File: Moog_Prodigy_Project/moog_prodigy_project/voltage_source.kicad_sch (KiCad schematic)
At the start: 19 parts, among them T1 230 VAC/ 15VAC 1.5A 22W, U24 L78L12, U25 L79L12

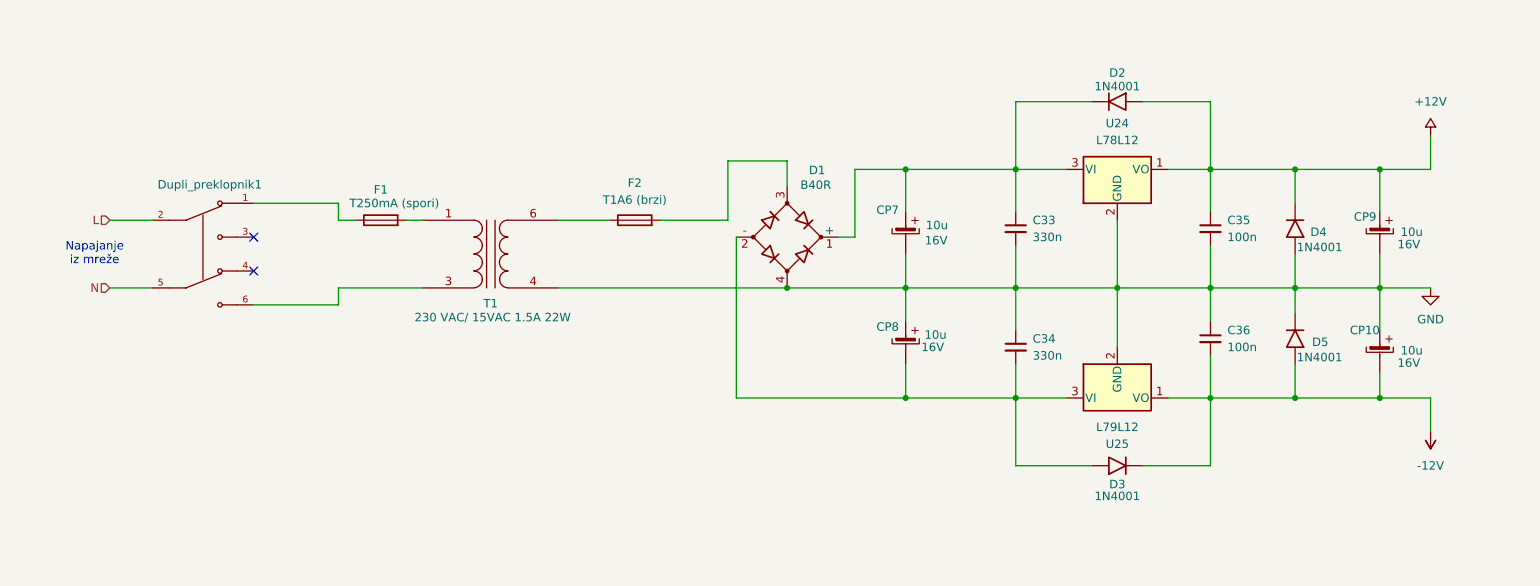
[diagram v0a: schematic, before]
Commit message: MOOG prodigy final 03.07.2026
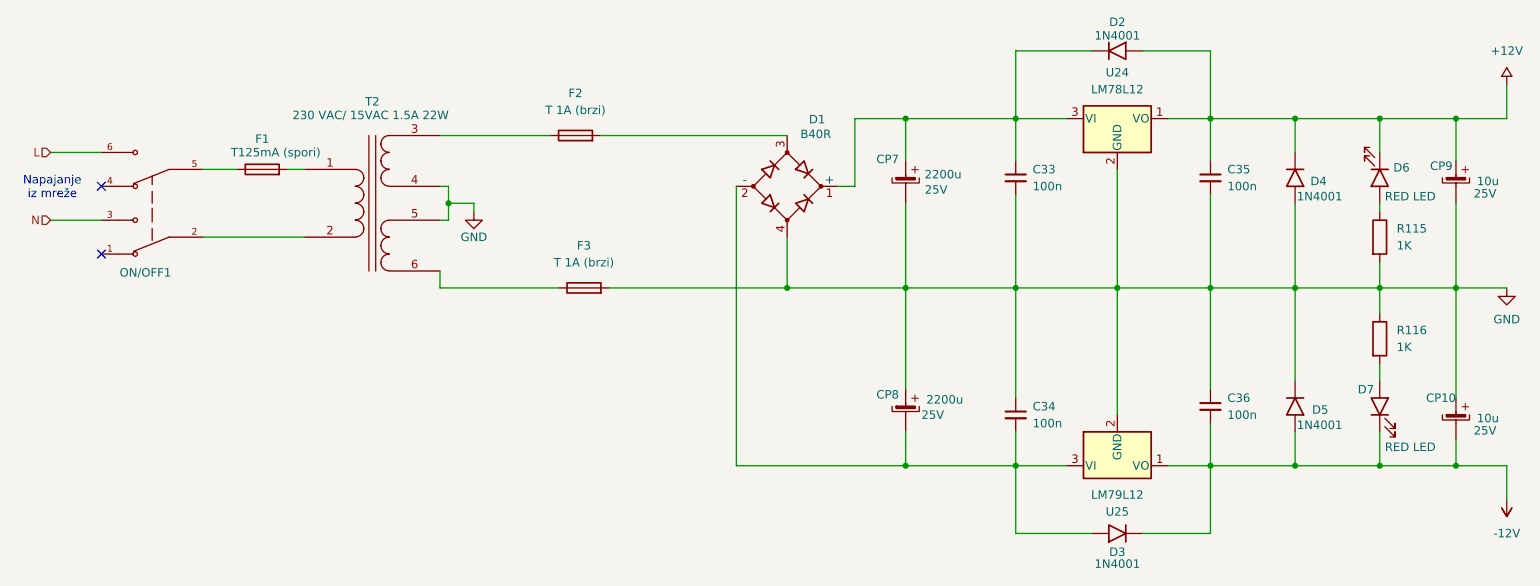
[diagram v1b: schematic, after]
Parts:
- removed T1: 230 VAC/ 15VAC 1.5A 22W, Transformer_THT:Transformer_NF_ETAL_P3324, symbol Device:Transformer_1P_1S
- added D6, D7: RED LED, symbol Device:LED
- added F3: T 1A (brzi), Fuse:Fuse_Bourns_MF-RHT100, symbol Device:Fuse
- added R115, R116: 1K, symbol Device:R
- added T2: 230 VAC/ 15VAC 1.5A 22W, Transformer_THT:Transformer_Myrra_EI30-5_44000_Horizontal, symbol Device:Transformer_1P_2S
- C33, C34: value 330n -> 100n
- CP10, CP9: Rated Voltage 16V -> 25V
- CP7, CP8: value 10u -> 2200u; Rated Voltage 16V -> 25V
- F1: value T250mA (spori) -> T125mA (spori)
- F2: value T1A6 (brzi) -> T 1A (brzi)
- U24: value L78L12 -> LM78L12
- U25: value L79L12 -> LM79L12
- renumbered Dupli_preklopnik1 to ON/OFF1
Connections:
- net +12V: now also D6.1 (K)
- net -12V: now also D7.1 (K)
- net GND: now also F3.2, R115.2, R116.1, T2.4 (SB), T2.5 (SC)
- net L: now also ON/OFF1.6; no longer ON/OFF1.2
- net N: now also ON/OFF1.3; no longer ON/OFF1.5
- net at ON/OFF1.1: no longer F1.1
- net at F1.2: now also T2.1 (AA)
- net at F2.1: now also T2.3 (SA)
- new net: ON/OFF1.2, T2.2 (AB)
- new net: F1.1, ON/OFF1.5
- new net: D6.2 (A), R115.1
- new net: D7.2 (A), R116.2
- new net: F3.1, T2.6 (SD)
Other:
- moved on the sheet: C33, C34, C35, C36, CP10, CP7, CP8, CP9, D1, D2, D3, D4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
